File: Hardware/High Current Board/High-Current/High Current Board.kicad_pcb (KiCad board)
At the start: 2 copper layers, 174.3 x 151.9 mm, 37 parts, among them J1 8P8C_Shielded, J2 Conn_01x04, J3 GND, J4 Load Resistors Return, J5 +46V from Fuel Cell, K1 G2RL-1A-E, K2 G2RL-1A-E, Q1 NMOS_Substrate, Q2 NMOS, U1 TC4421AVAT, U3 HO 25-P

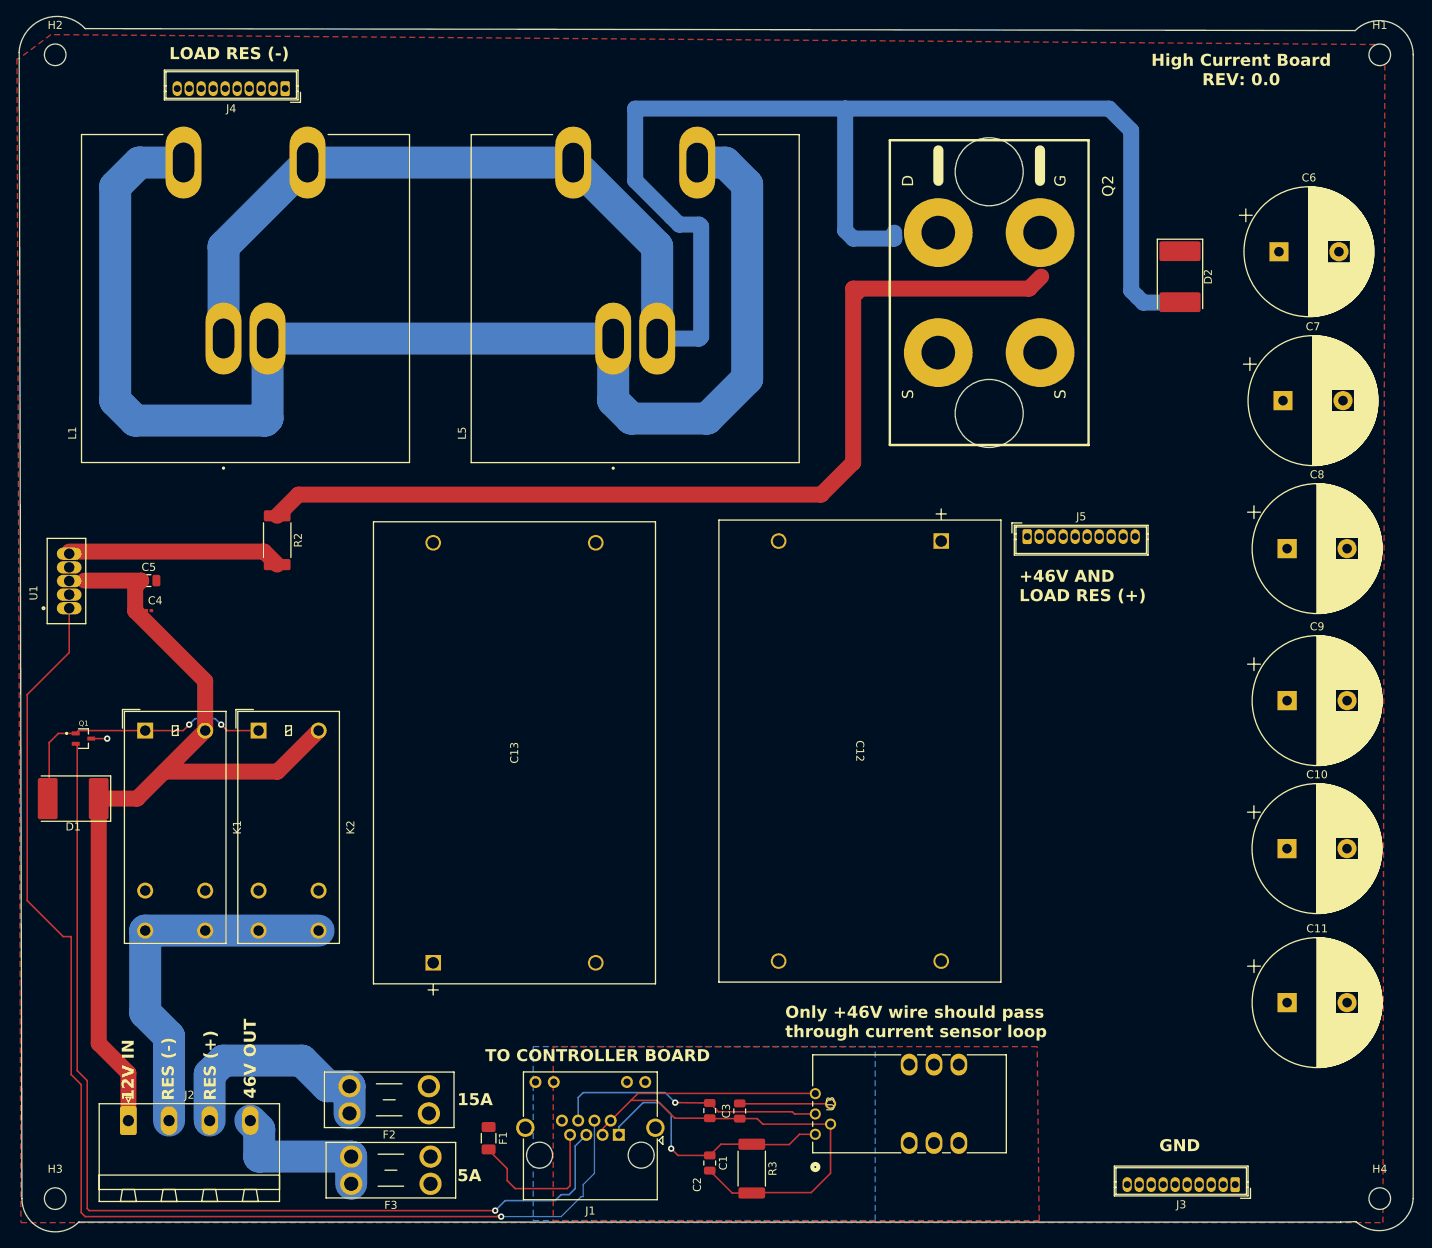
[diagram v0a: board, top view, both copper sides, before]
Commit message: PCB Update - HC
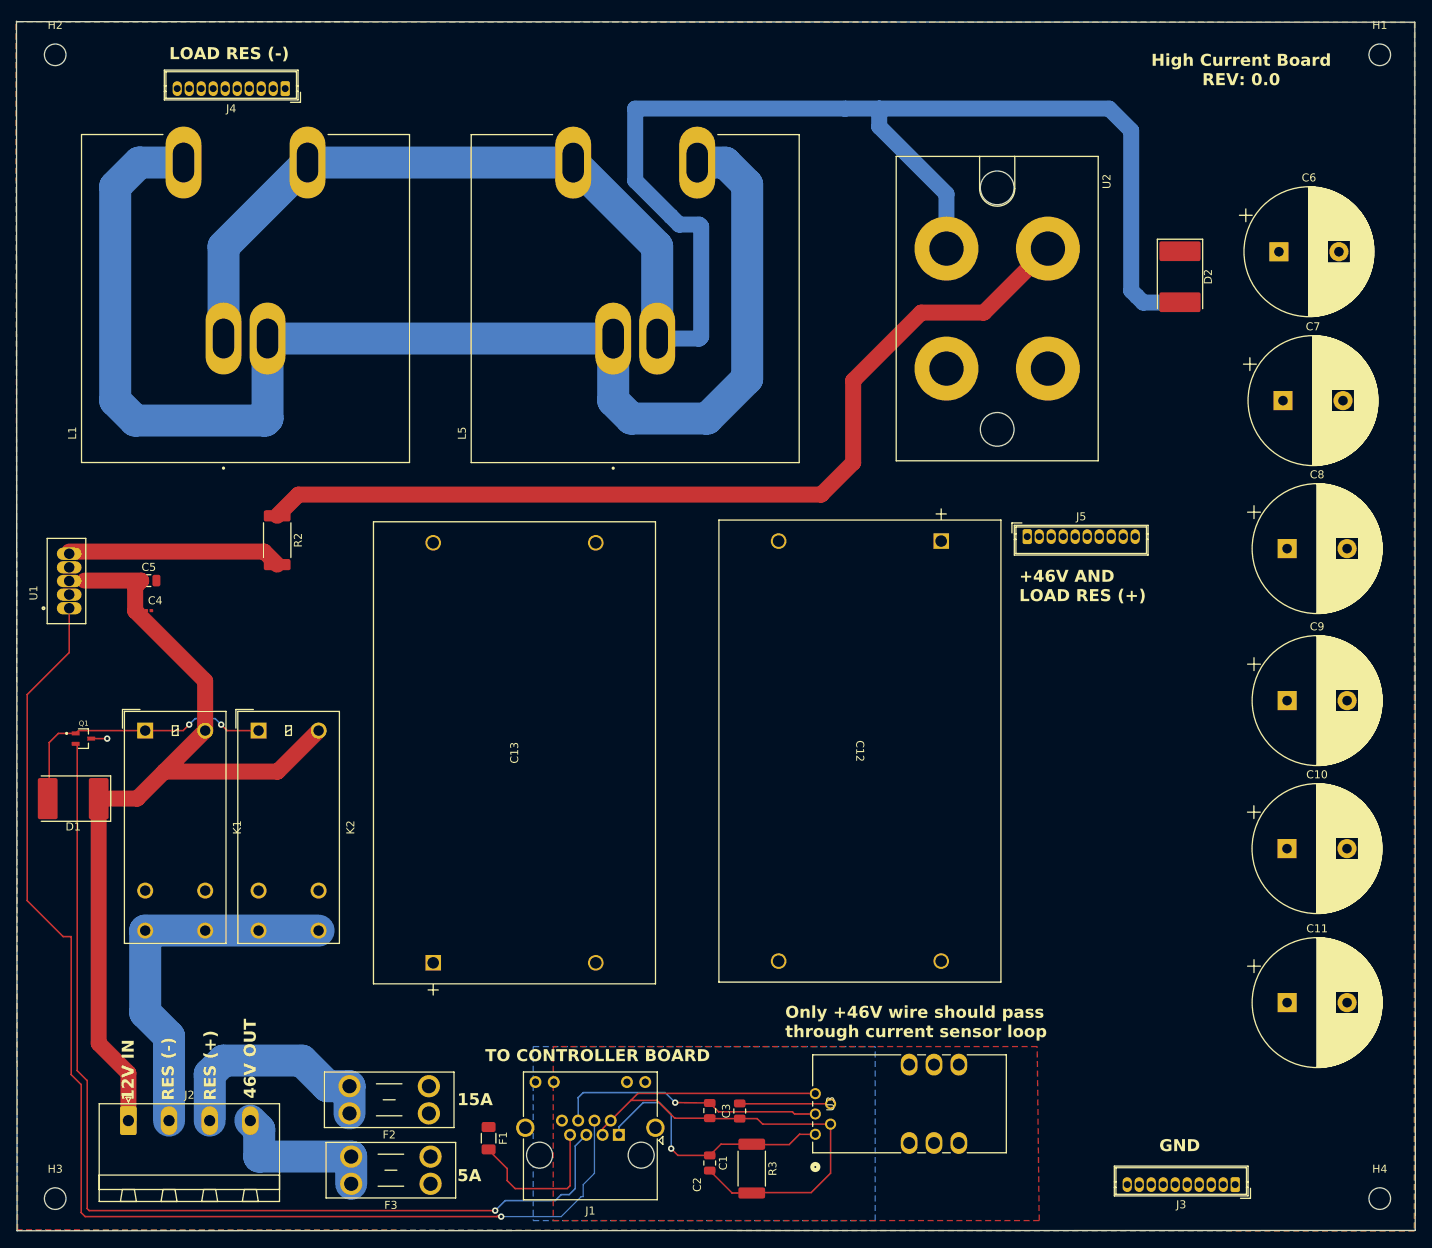
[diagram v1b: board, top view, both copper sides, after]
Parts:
- removed Q2: NMOS, KiCADv6:SOT-227B
- added U2: ~, KiCADv6:GENESIC_MBR200100CTS, F.Cu at (167.8, 51.8)
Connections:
- R2 pad 1: Net-(Q2-D) -> GATE_DRIVE
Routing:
- net Net-(Q2-D): track 120.8 -> 0.00 mm
- net GATE_DRIVE: track 0.00 -> 116.2 mm
- net Net-(D2-A): track 237.2 -> 235.6 mm
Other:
- board size 174.3 x 151.9 mm -> 174.9 x 151.1 mm
